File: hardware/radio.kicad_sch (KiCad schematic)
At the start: 59 parts, among them J1 105450-0101, J2 Conn_01x02, J3 Conn_01x02, J4 Conn_01x04, J5 Conn_01x02_Male, Q1 Q_PMOS_DGS, Q2 Q_NMOS_DGS, Q3 Q_NMOS_DGS, Q4 Q_PMOS_DGS, SW1 SW_BOOT, SW2 SW_RST, SW3 SW_1, SW4 Rot_Enc, SW5 SW_2, SW6 SW_3, U1 TP4056, U2 ESP32-WROOM-32, U3 TPS5432, U4 MAX98357

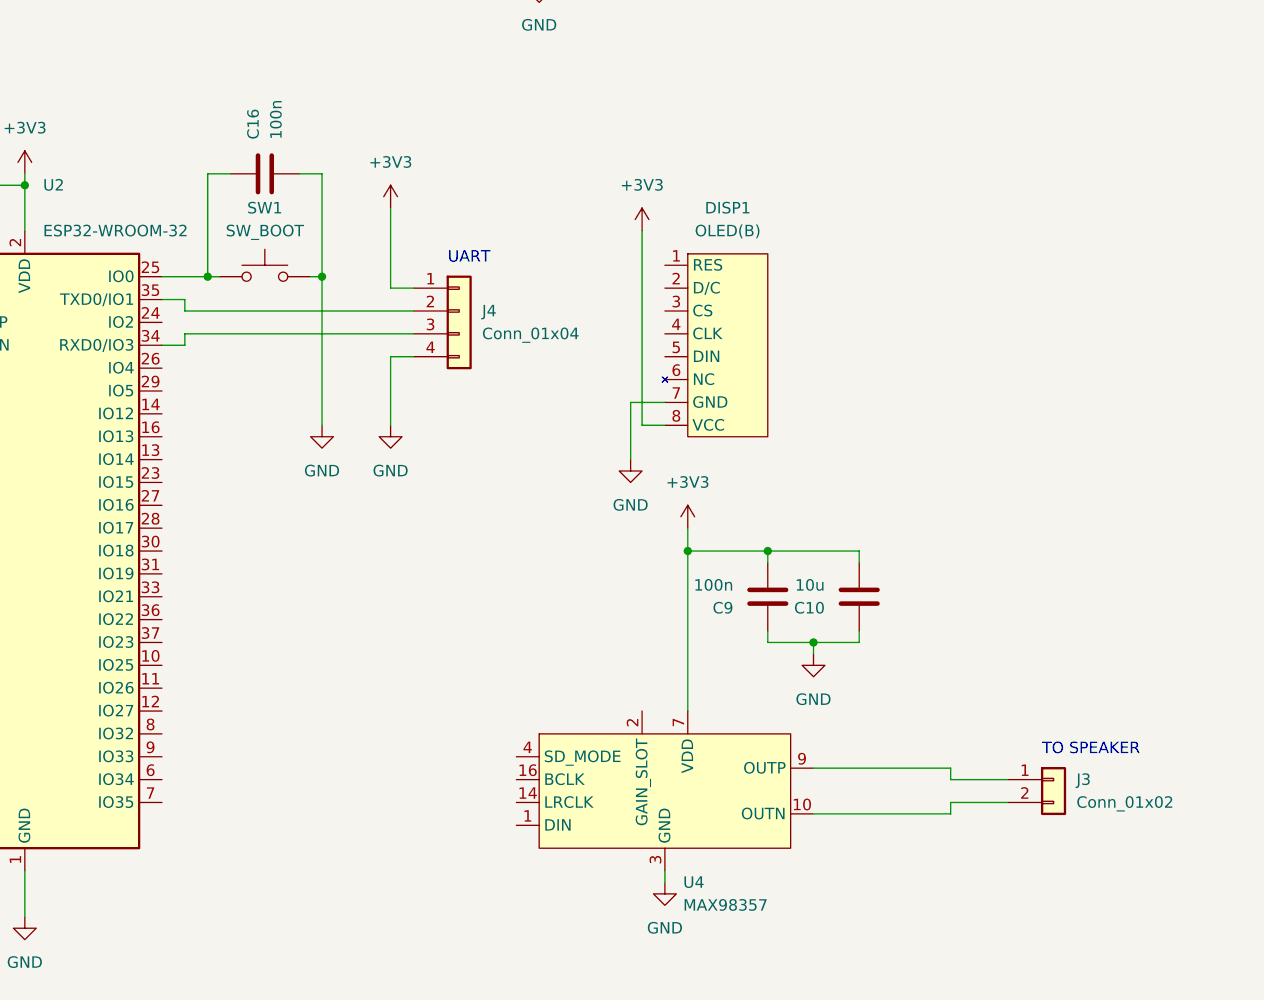
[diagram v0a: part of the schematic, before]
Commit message: routing
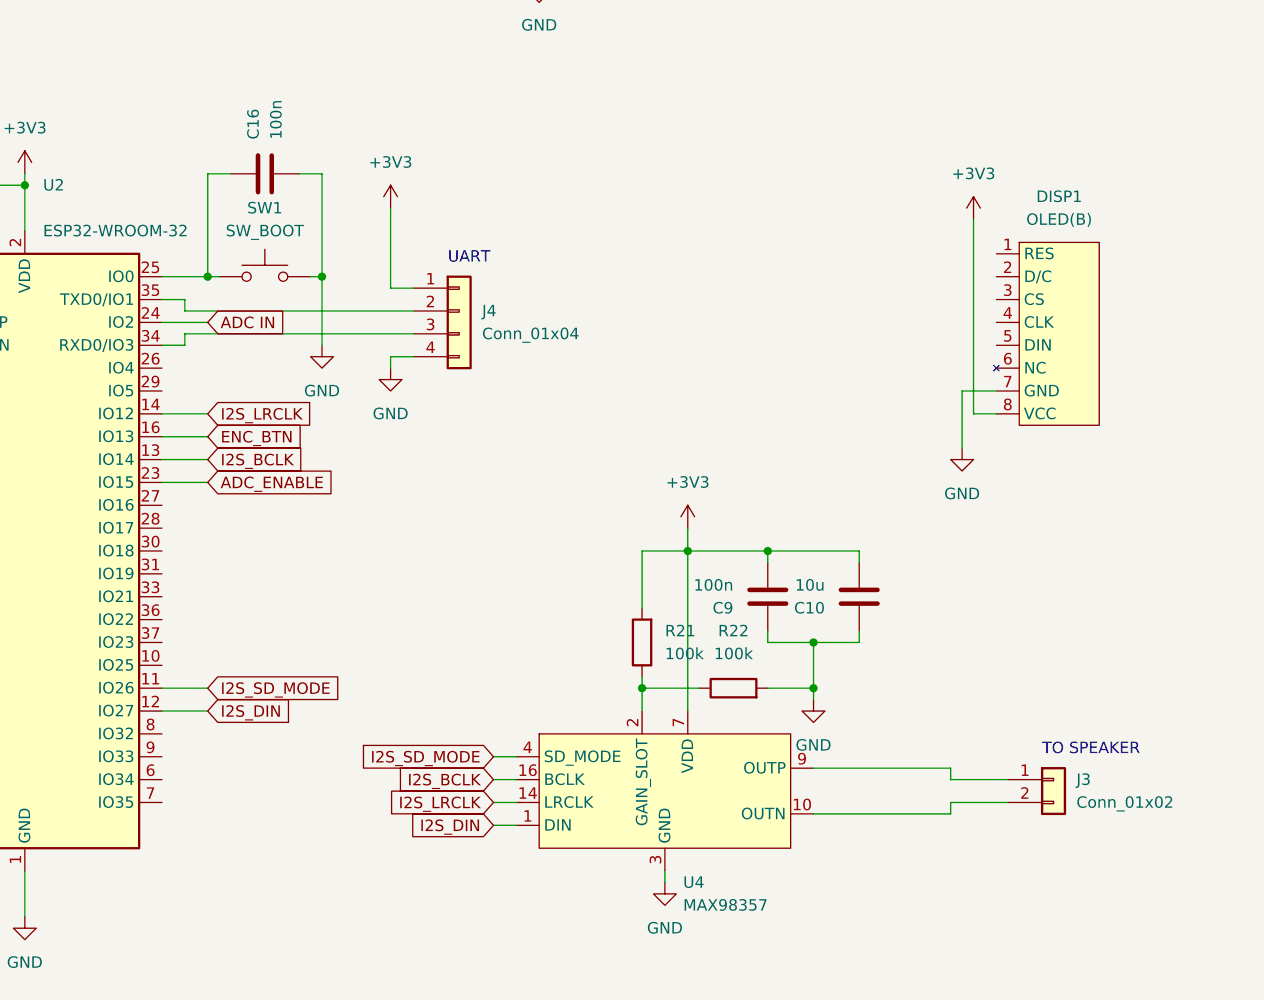
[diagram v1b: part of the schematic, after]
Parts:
- added R21, R22: 100k, Resistor_SMD:R_0603_1608Metric, symbol Device:R
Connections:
- net +3V3: now also R21.2
- net ADC IN: now also U2.24 (IO2)
- net ADC_ENABLE: now also U2.23 (IO15)
- net ENC_BTN: now also U2.16 (IO13)
- net GND: now also R22.2
- net I2S_DIN: now reaches U4.1 (DIN)
- net I2S_DIN: now also U2.12 (IO27)
- net I2S_LRCLK: now reaches U4.14 (LRCLK)
- net I2S_LRCLK: now also U2.14 (IO12)
- net I2S_BCLK: now reaches U4.16 (BCLK)
- net I2S_BCLK: now also U2.13 (IO14)
- net at U4.2 (GAIN_SLOT): now also R21.1, R22.1
- net I2S_SD_MODE: now reaches U4.4 (SD_MODE)
- net I2S_SD_MODE: now also U2.11 (IO26)
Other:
- moved on the sheet: DISP1
